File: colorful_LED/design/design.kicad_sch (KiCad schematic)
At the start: 25 parts, among them J1 USB_B, SW1 SW_Push, SW2 SW_Wuerth_450301014042, U1 ATmega32U4-A, Y1 8MHz

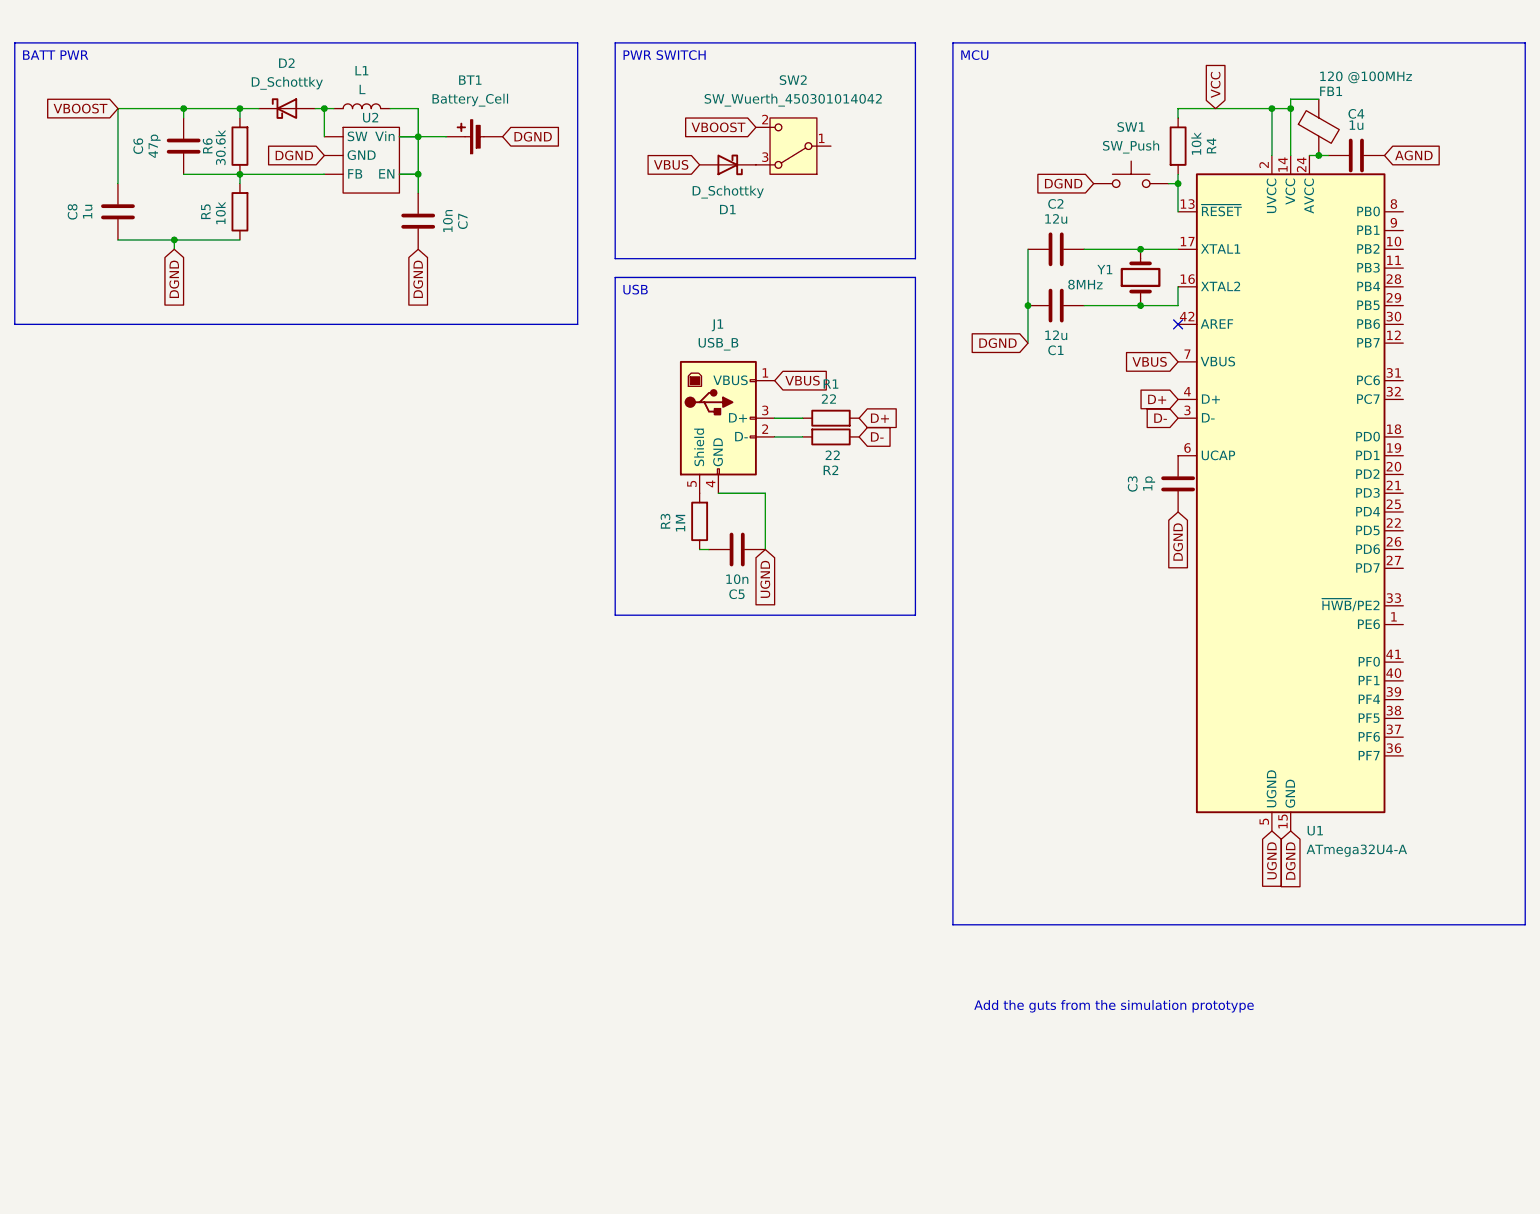
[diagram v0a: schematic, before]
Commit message: Finished analog
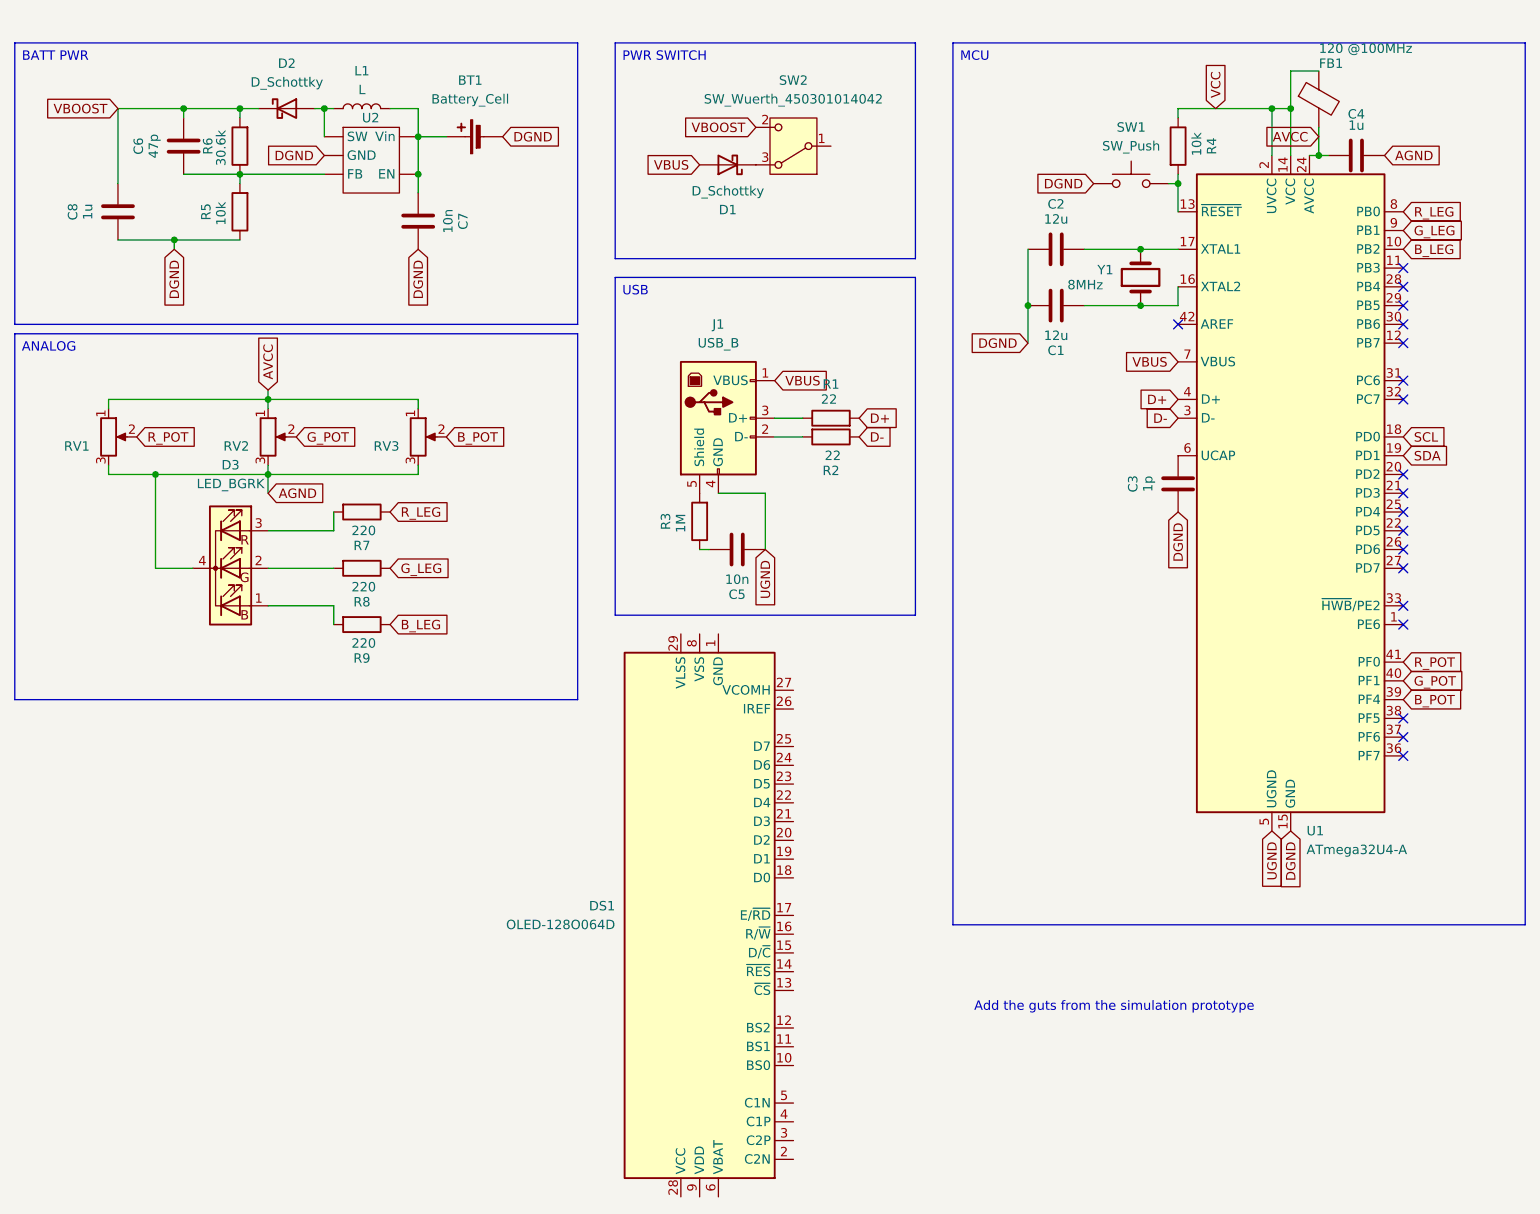
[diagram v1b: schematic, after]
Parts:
- added D3: LED_BGRK, symbol Device:LED_BGRK
- added DS1: OLED-128O064D, Display:OLED-128O064D, symbol Display_Graphic:OLED-128O064D
- added R7, R8, R9: 220, Resistor_SMD:R_0805_2012Metric, symbol Device:R
- added RV1, RV2, RV3: R_Potentiometer, Potentiometer_SMD:Potentiometer_ACP_CA6-VSMD_Vertical, symbol Device:R_Potentiometer
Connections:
- net AGND: now also D3.4 (K), RV1.3, RV2.3, RV3.3
- net AVCC: now reaches C4.2, FB1.2, U1.24 (AVCC), U1.44 (AVCC)
- net AVCC: now also RV1.1, RV2.1, RV3.1
- net B_LEG: now reaches U1.10 (PB2)
- net B_LEG: now also R9.1
- net SCL: now reaches U1.18 (PD0)
- net SDA: now reaches U1.19 (PD1)
- net B_POT: now reaches U1.39 (PF4)
- net B_POT: now also RV3.2
- net G_POT: now reaches U1.40 (PF1)
- net G_POT: now also RV2.2
- net R_POT: now reaches U1.41 (PF0)
- net R_POT: now also RV1.2
- net R_LEG: now reaches U1.8 (PB0)
- net R_LEG: now also R7.1
- net G_LEG: now reaches U1.9 (PB1)
- net G_LEG: now also R8.1
- new net: D3.2 (GA), R8.2
- new net: D3.3 (RA), R7.2
- new net: DS1.1 (GND), DS1.30 (GND)
- new net: D3.1 (BA), R9.2
- no-connect marks 1 -> 19
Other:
- moved on the sheet: FB1

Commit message: Finished Schematic
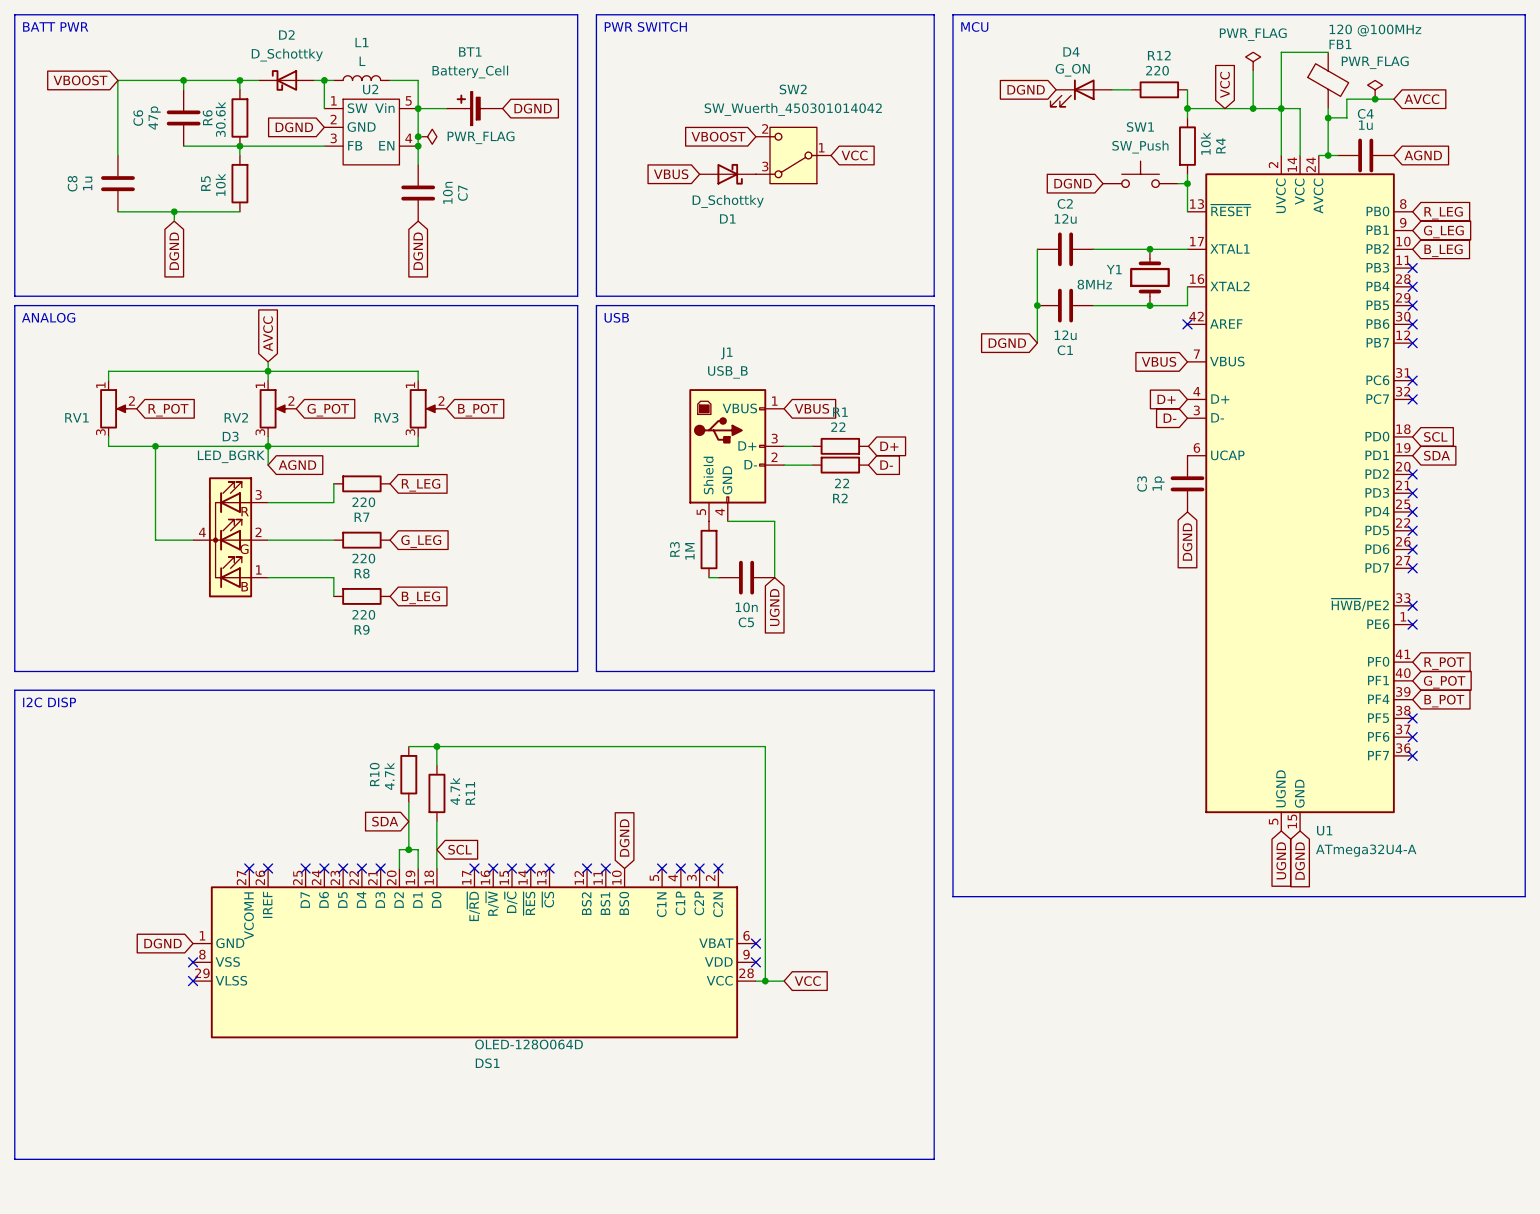
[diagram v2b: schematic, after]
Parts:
- added D4: G_ON, LED_SMD:LED_0805_2012Metric, symbol Device:LED
- added R10, R11: 4.7k, Resistor_SMD:R_0805_2012Metric, symbol Device:R
- added R12: 220, Resistor_SMD:R_0805_2012Metric, symbol Device:R
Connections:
- net DGND: now also DS1.1 (GND), DS1.10 (BS0), DS1.30 (GND), U2.2 (GND), D4.1 (K); no longer U2. (EN)
- net SCL: now also DS1.18 (D0), R11.2
- net SDA: now also DS1.19 (D1), DS1.20 (D2), R10.1
- net VCC: now also DS1.28 (VCC), SW2.1 (B), R10.2, R11.1, R12.2
- net at C6.2, R5.2, R6.1: now also U2.3 (FB); no longer U2. (EN)
- net at D2.2 (A), L1.1: now also U2.1 (SW); no longer U2. (EN)
- net at BT1.1 (+), C7.2, L1.2: now also U2.4 (EN), U2.5 (Vin); no longer U2. (EN)
- new net: D4.2 (A), R12.1
- no-connect marks 19 -> 41
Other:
- note removed: "Add the guts from the simulation prototype"
- moved on the sheet: BT1, C1, C2, C3, C4, C5, C6, C7, C8, D1, D2, D3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
